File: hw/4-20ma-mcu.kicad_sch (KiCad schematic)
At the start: 4 parts, among them U1 ATtiny84A-SS, U2 LM324A

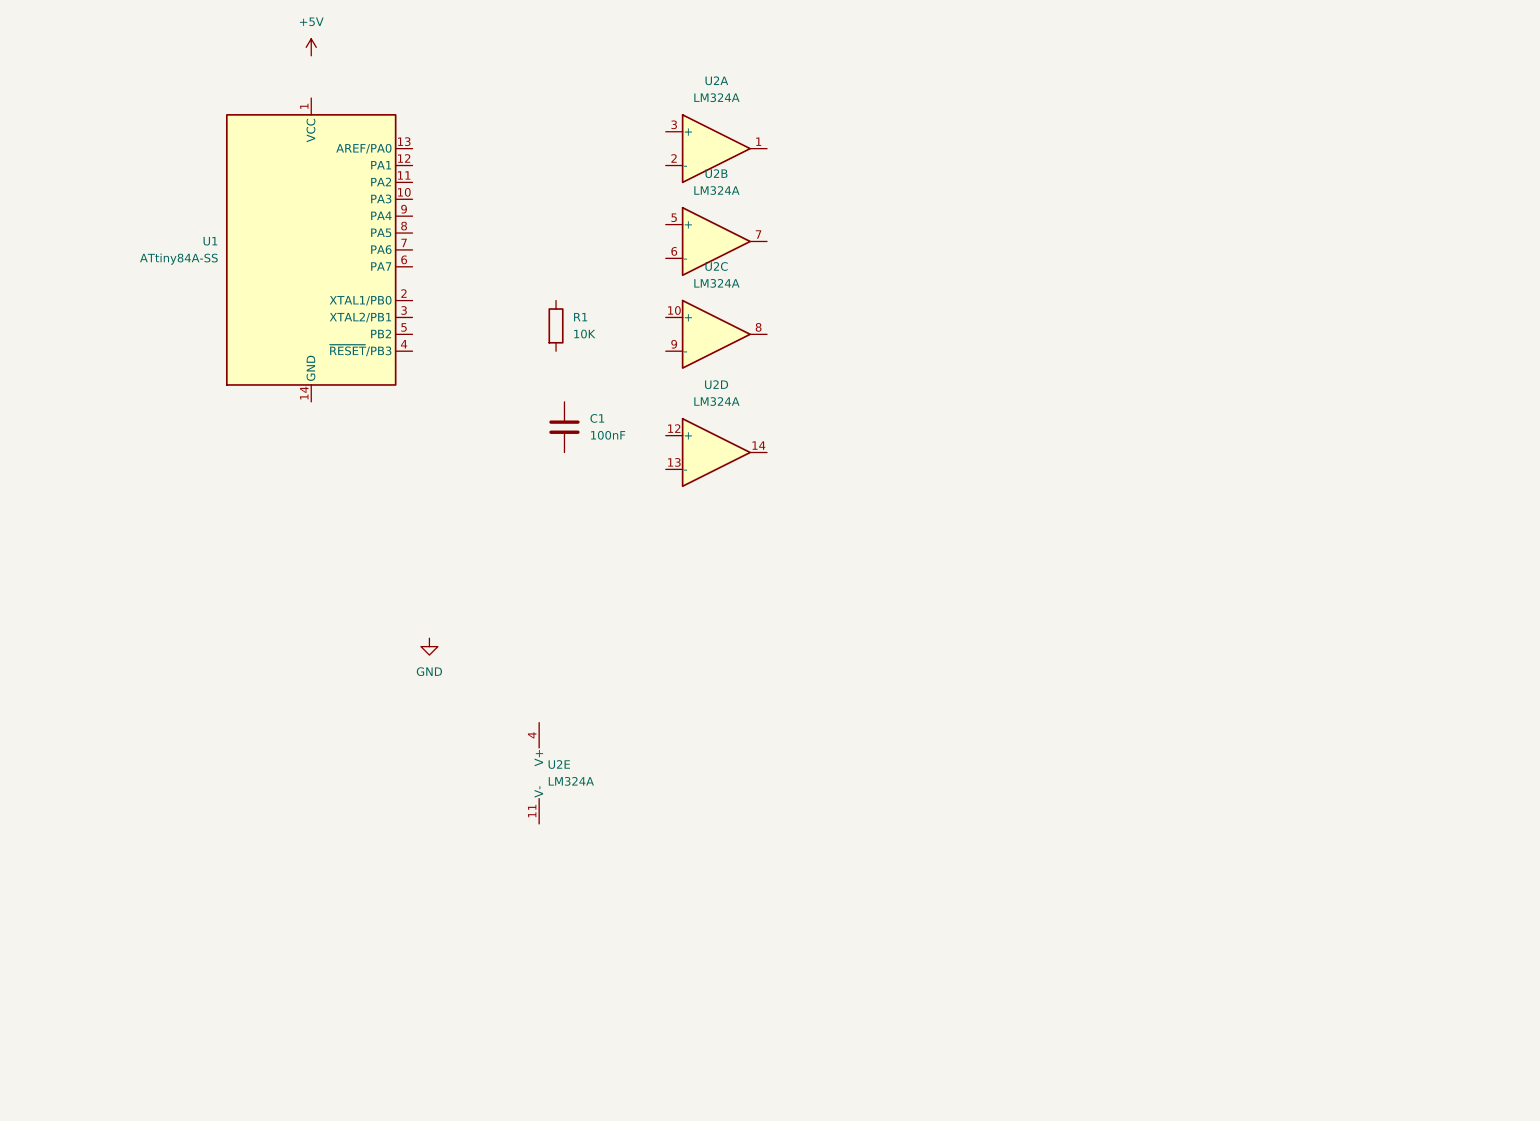
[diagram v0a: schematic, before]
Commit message: dev update 030425
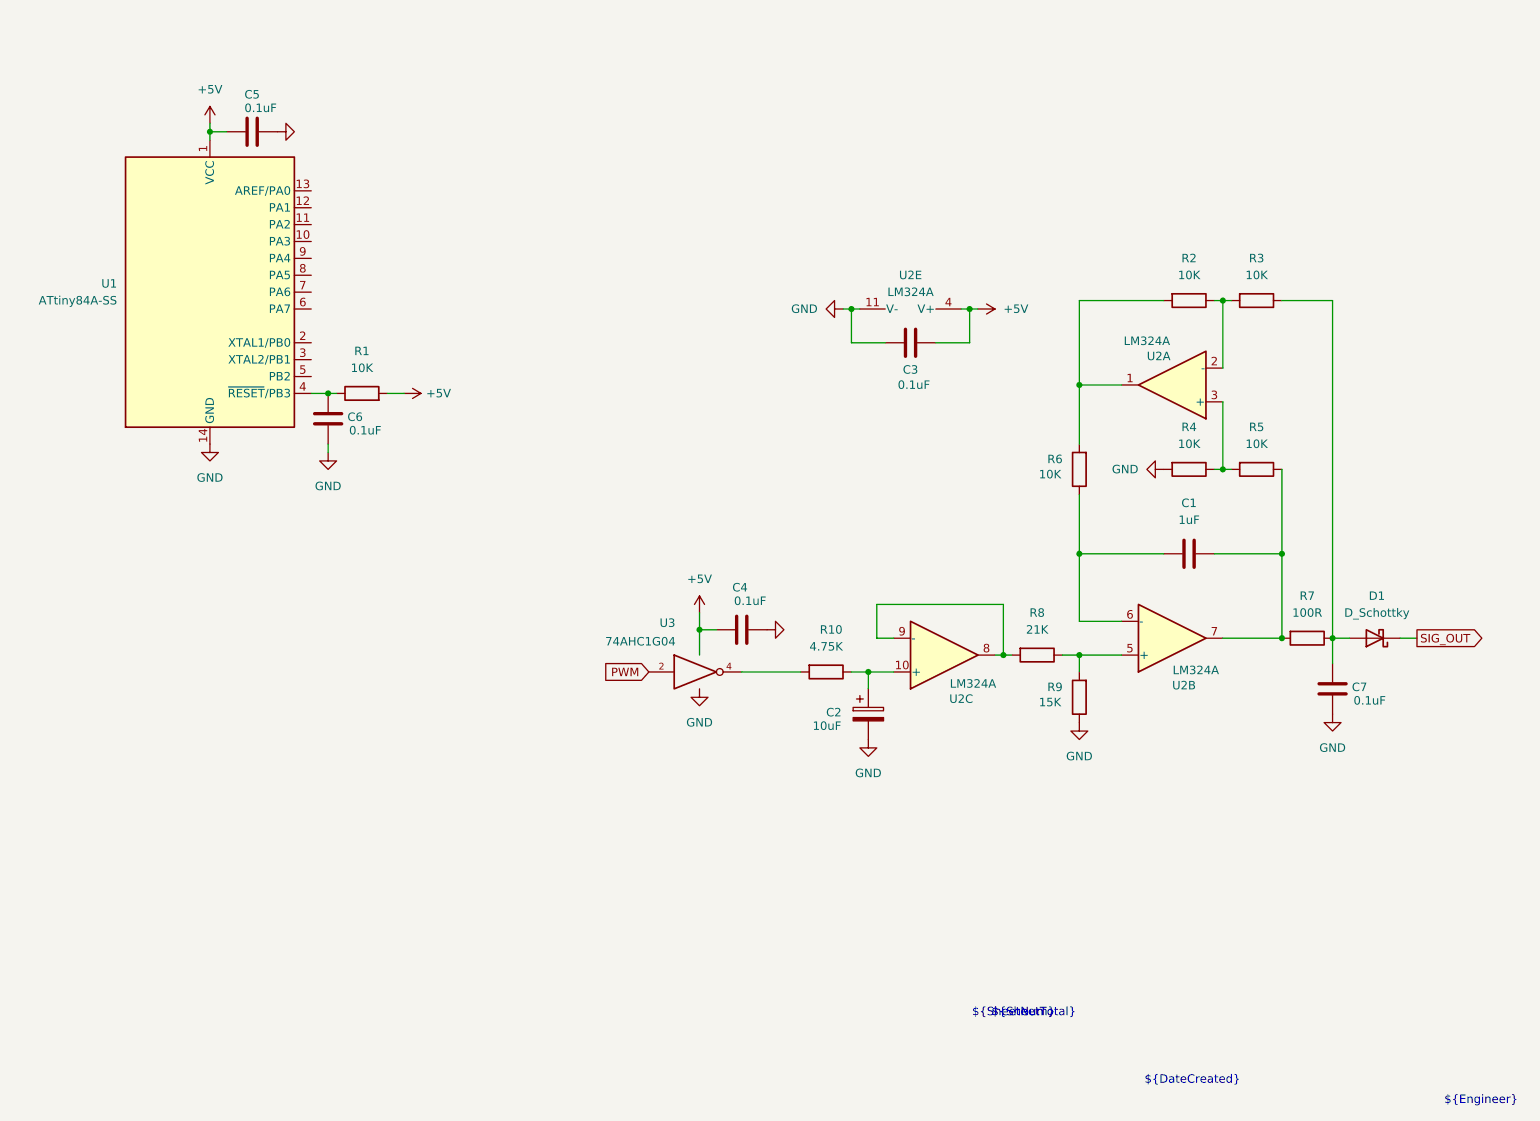
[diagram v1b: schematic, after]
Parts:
- removed unit 4 of U2
- added C2: 10uF, Capacitor_SMD:C_1206_3216Metric, symbol Device:C_Polarized
- added C3, C4, C5, C6, C7: 0.1uF, Capacitor_SMD:C_0805_2012Metric, symbol Device:C
- added D1: D_Schottky, Package_TO_SOT_SMD:SOT-23, symbol Device:D_Schottky
- added R10: 4.75K, R_0805_2012Metric, symbol Device:R
- added R2, R3, R4, R5, R6: 10K, R_0805_2012Metric, symbol Device:R
- added R7: 100R, R_0805_2012Metric, symbol Device:R
- added R8: 21K, R_0805_2012Metric, symbol Device:R
- added R9: 15K, R_0805_2012Metric, symbol Device:R
- added U3: 74AHC1G04, Package_TO_SOT_SMD:SOT-23-5, symbol 74xGxx:74AHC1G04
- C1: value 100nF -> 1uF; footprint C_0805_2012Metric_Pad1.18x1.45mm_HandSolder -> Capacitor_SMD:C_0805_2012Metric
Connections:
- net +5V: now also R1.2, U1.1 (VCC), U2.4 (V+), C3.1, C4.2, C5.2, U3.5 (VCC)
- net GND: now also U1.14 (GND), U2.11 (V-), C2.2, C3.2, C4.1, C5.1, C6.2, C7.2, R4.2, R9.1, U3.3 (GND)
- net at U2.1: now also R2.2, R6.2
- net at U2.2 (-): now also R2.1, R3.2
- net at U2.3 (+): now also R4.1, R5.2
- net at U2.5 (+): now also R8.1, R9.2
- net at U2.6 (-): now also C1.2, R6.1
- net at U2.7: now also C1.1, R5.1, R7.2
- net at U2.10 (+): now also C2.1, R10.1
- net at U2.8: now also U2.9 (-), R8.2
- net at R1.1: now also U1.4 (~{RESET}/PB3), C6.1
- new net: C7.1, D1.2 (A), R3.1, R7.1
- new net: R10.2, U3.4
- new net PWM: U3.2
- new net SIG_OUT: D1.1 (K)
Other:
- note added: "${DateCreated}"
- note added: "${Engineer}"
- note added: "${Revision}"
- note added: "${SheetNum}"
- note added: "${SheetTotal}"
- note added: "${Title}"
- moved on the sheet: C1, R1, U1, U2A, U2B, U2C, U2E
